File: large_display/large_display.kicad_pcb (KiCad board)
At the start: 2 copper layers, 128 parts, among them J1 Conn_01x11, J2 Conn_01x11, U1 TLC5940PWP

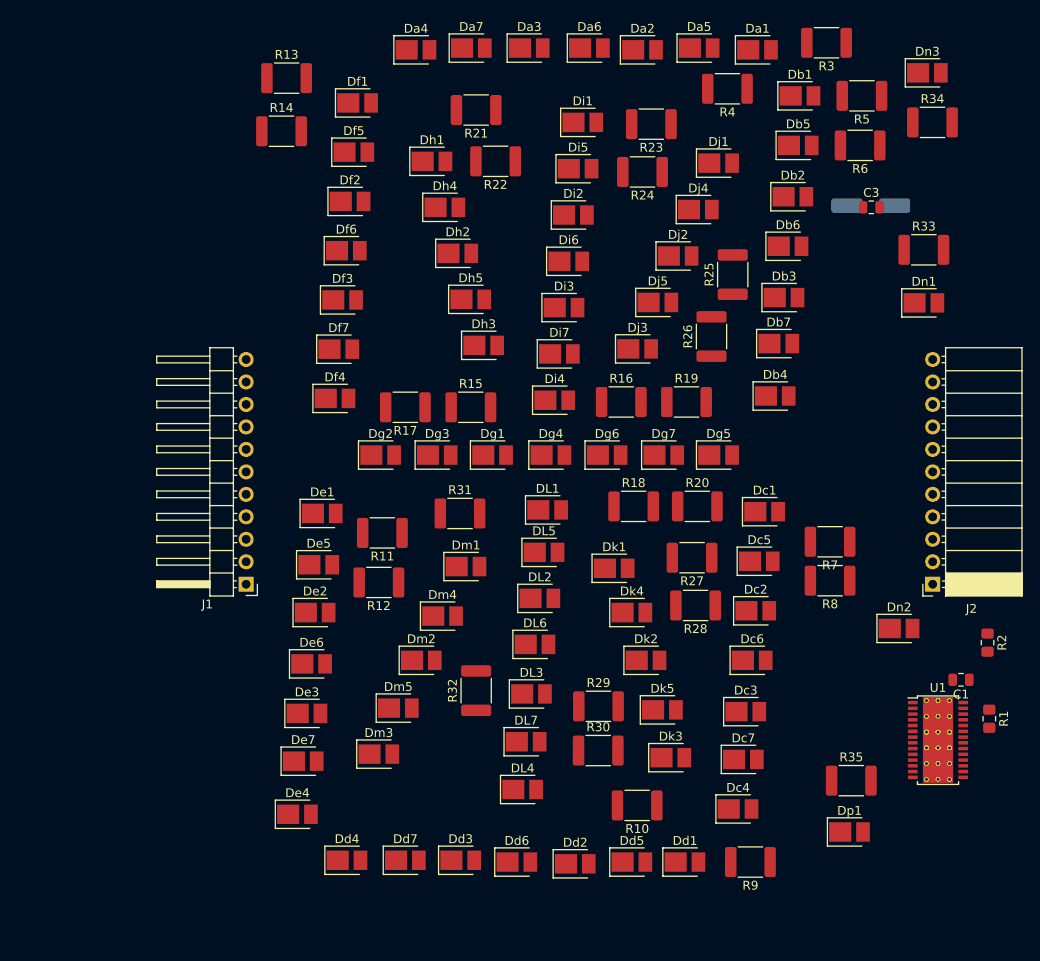
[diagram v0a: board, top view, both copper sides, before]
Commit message: routing: first pass done
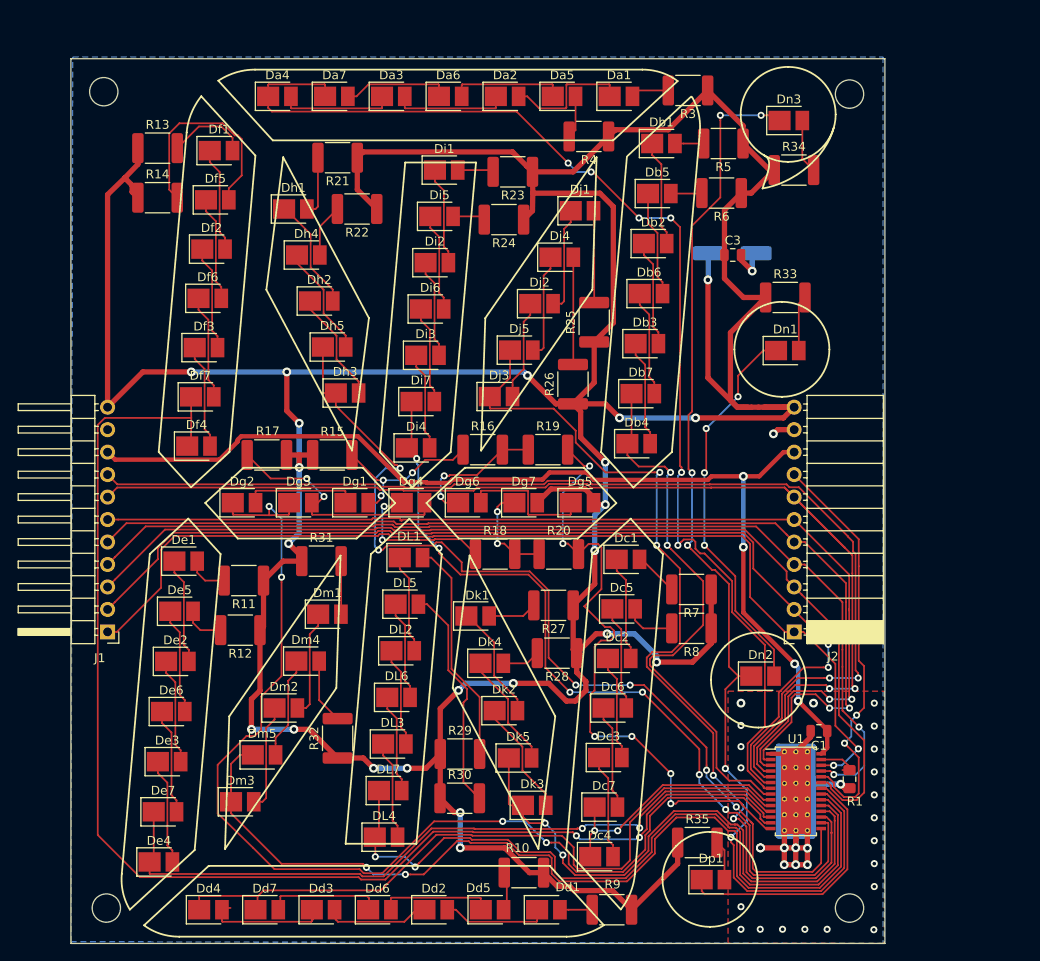
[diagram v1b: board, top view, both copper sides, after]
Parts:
- removed R2: R, Resistor_SMD:R_0805_2012Metric_Pad1.15x1.40mm_HandSolder
- added REF**: MountingHole_3.2mm_M3, MountingHole:MountingHole_3.2mm_M3, F.Cu at (138.4, 146.8)
- added REF**: MountingHole_3.2mm_M3, MountingHole:MountingHole_3.2mm_M3, F.Cu at (54.0, 146.0)
- added REF**: MountingHole_3.2mm_M3, MountingHole:MountingHole_3.2mm_M3, F.Cu at (138.2, 53.8)
- added REF**: MountingHole_3.2mm_M3, MountingHole:MountingHole_3.2mm_M3, F.Cu at (53.7, 53.7)
- moved R35 18.8 mm to (120.8, 138.6)
- moved R1 17.2 mm to (138.0, 131.4)
- moved Dk5 17.2 mm to (100.5, 129.0)
- moved U1 17.1 mm to (131.9, 132.8)
- moved C1 17.1 mm to (134.5, 126.0)
- moved Dk4 17.1 mm to (97.3, 118.3)
- moved Dk2 17.0 mm to (98.9, 123.7)
- moved Dd5 16.9 mm to (97.4, 146.2)
- moved Da6 16.9 mm to (92.6, 54.3)
- moved Dd7 16.8 mm to (71.9, 146.2)
- moved De7 16.8 mm to (60.4, 135.1)
- moved Db5 16.8 mm to (116.3, 65.2)
- moved Dd2 16.8 mm to (91.0, 146.2)
- moved DL2 16.8 mm to (87.3, 116.9)
- moved DL5 16.8 mm to (87.7, 111.7)
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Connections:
- Df7 pad 1: Net-(Df7-Pad1) -> Net-(Df4-Pad1)
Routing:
- net Vdrive: track 0.00 -> 494.7 mm, vias 0 -> 22
- net Net-(Df4-Pad1): track 0.00 -> 148.1 mm, vias 0 -> 2
- net Net-(Da4-Pad1): track 0.00 -> 134.8 mm, vias 0 -> 6
- net Net-(J1-Pad7): track 0.00 -> 132.7 mm, vias 0 -> 2
- net Net-(Dg2-Pad1): track 0.00 -> 126.5 mm, vias 0 -> 4
- net Net-(Dn2-Pad1): track 0.00 -> 126.1 mm, vias 0 -> 6
- net Net-(J1-Pad8): track 0.00 -> 125.0 mm, vias 0 -> 2
- net VCC: track 0.00 -> 119.1 mm, vias 0 -> 4
- net Net-(J1-Pad6): track 0.00 -> 119.0 mm, vias 0 -> 2
- net Net-(J1-Pad5): track 0.00 -> 118.1 mm, vias 0 -> 2
- net Net-(J1-Pad3): track 0.00 -> 116.5 mm
- net Net-(J1-Pad2): track 0.00 -> 115.2 mm, vias 0 -> 2
- net Net-(J1-Pad1): track 0.00 -> 114.7 mm, vias 0 -> 2
- net Net-(J1-Pad4): track 0.00 -> 113.6 mm, vias 0 -> 2
- net Net-(Dh3-Pad1): track 0.00 -> 110.0 mm, vias 0 -> 6
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- added copper zone on B.Cu, net GND
- added copper zone on F.Cu, net GND
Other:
- board outline added: 92 x 100 mm
- net class Default: clearance 0.2 -> 0.16; trace_width 0.25 -> 0.2
- net class HiPower added: clearance 0.16, trace_width 0.6, via_dia 1, via_drill 0.5
- net class Lowpower added: clearance 0.16, trace_width 0.5, via_dia 1, via_drill 0.5
- rule trace_clearance: 0.2 -> 0.16
- board text added: "VLED GND VCC SDO SCK"
